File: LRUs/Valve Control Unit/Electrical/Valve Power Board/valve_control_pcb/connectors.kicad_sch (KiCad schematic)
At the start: 21 parts, among them J7 0768290110, J8 Conn_02x10_Odd_Even, U7 TPD6E05U06RVZ, U8 TPD6E05U06RVZ, U9 PCA9306DC

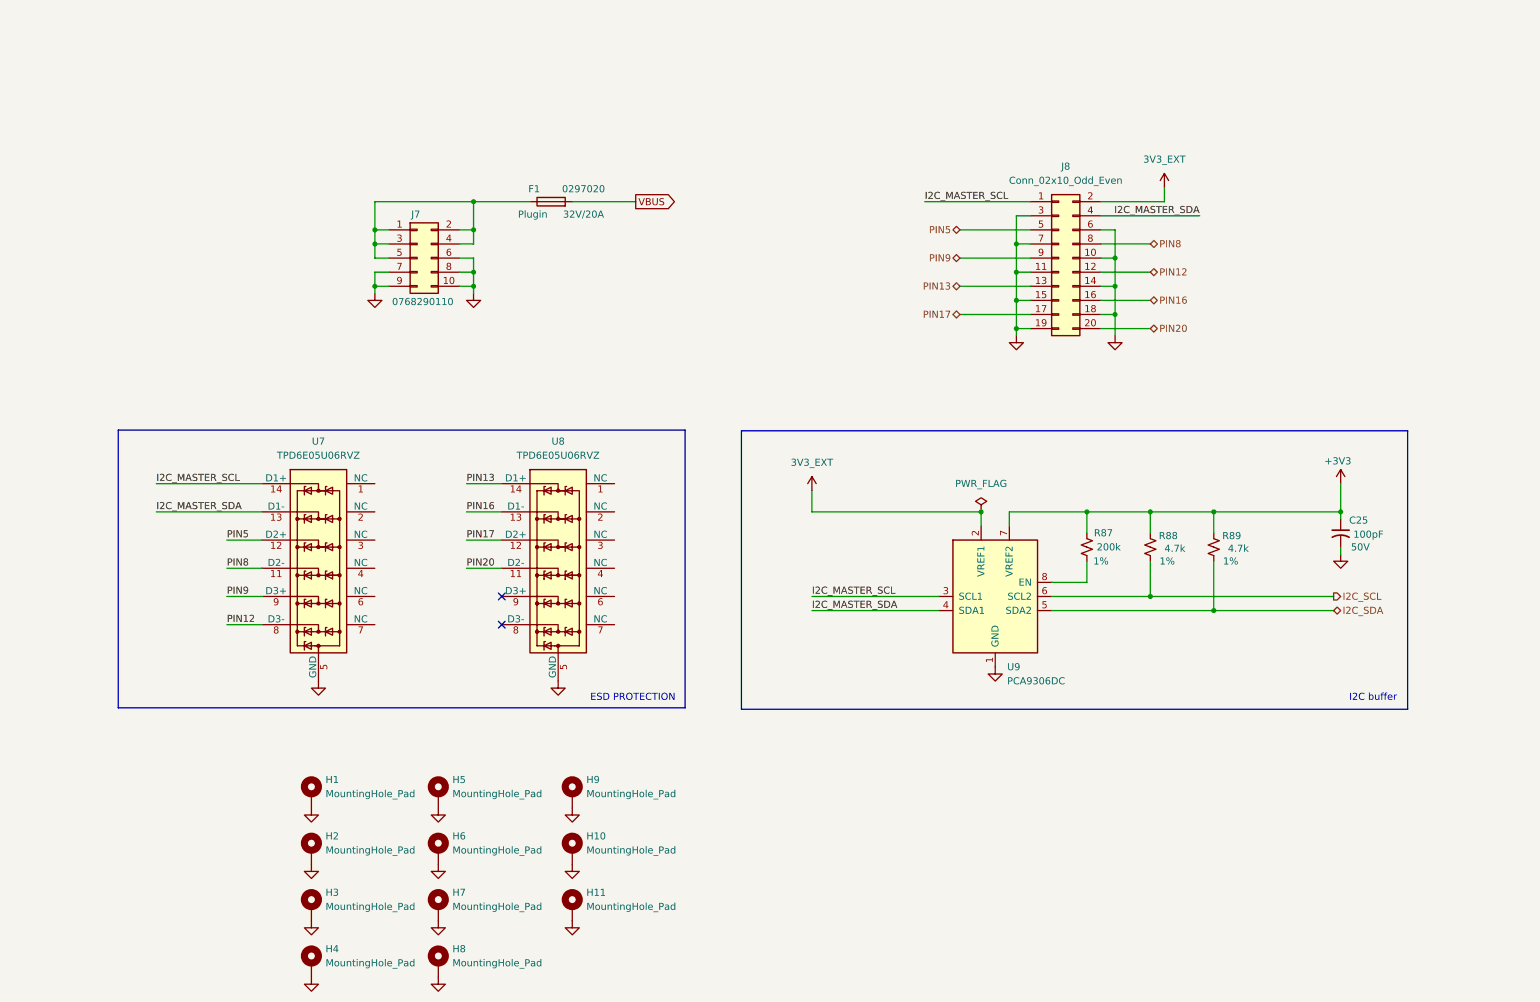
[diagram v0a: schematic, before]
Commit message: Commit valve board updates
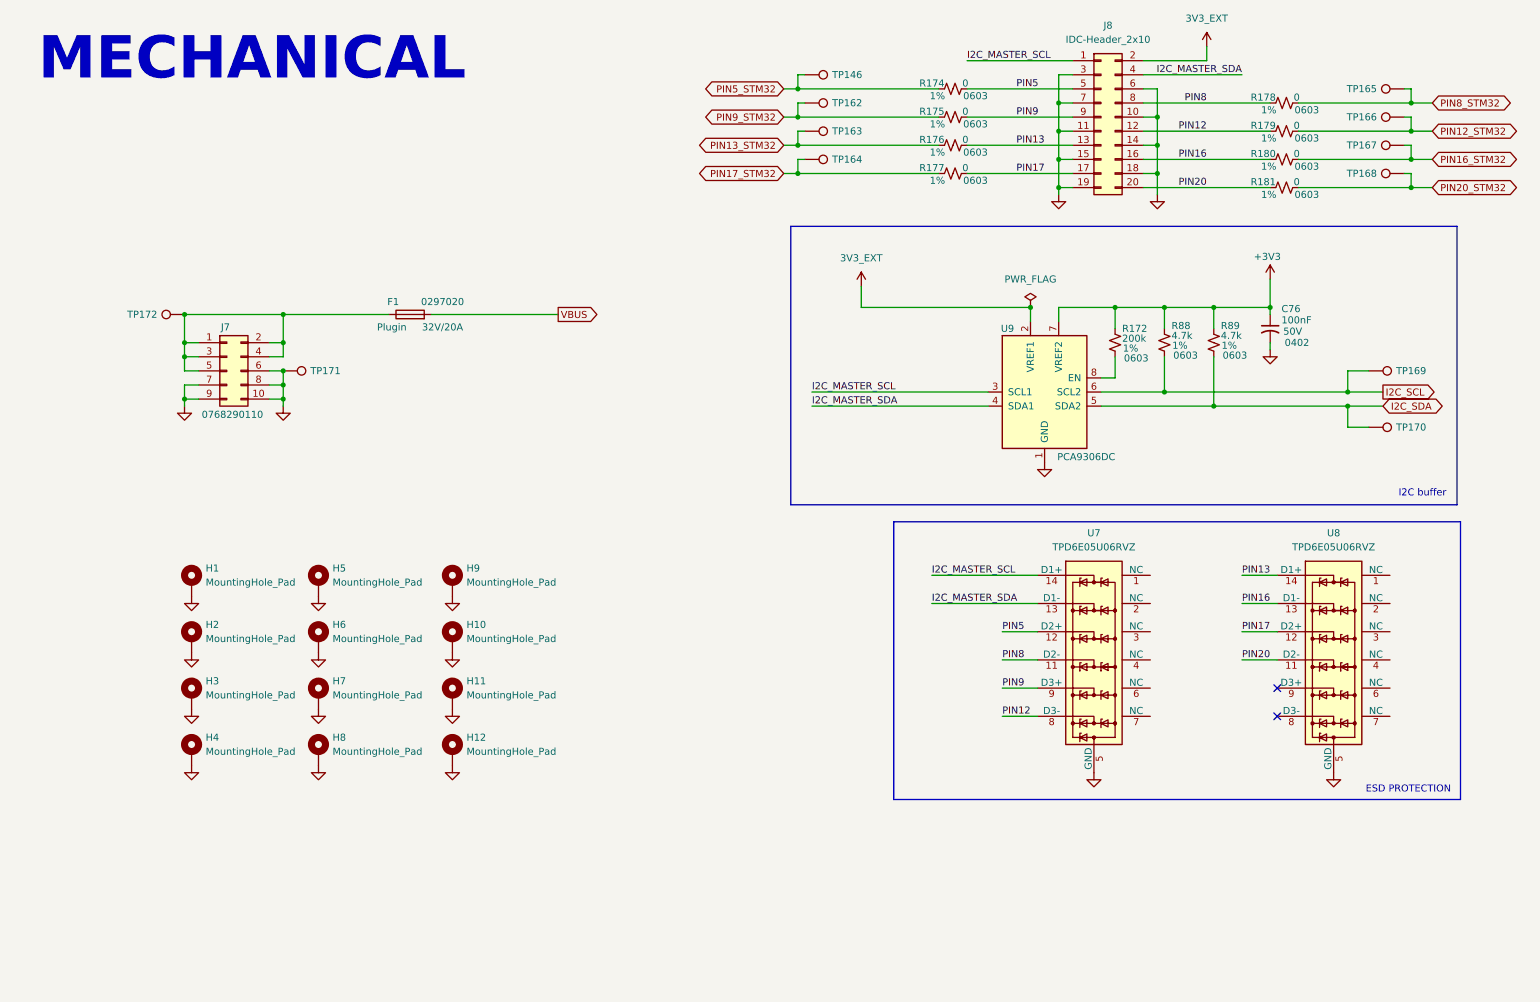
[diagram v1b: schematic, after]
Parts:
- removed C25: 100pF, Capacitor_SMD:C_0402_1005Metric, symbol Device:C_Small_US
- removed R87: 200k, Resistor_SMD:R_0603_1608Metric, symbol Device:R_Small_US
- added C76: 100nF, Capacitor_SMD:C_0402_1005Metric, symbol Device:C_Small_US
- added H12: MountingHole_Pad, MountingHole:MountingHole_3.2mm_M3_ISO14580_Pad, symbol Mechanical:MountingHole_Pad
- added R172: 200k, Resistor_SMD:R_0603_1608Metric, symbol Device:R_Small_US
- added R174, R175, R176, R177, R178, R179, R180, R181: 0, Resistor_SMD:R_0603_1608Metric, symbol Device:R_Small_US
- added TP146, TP162, TP163, TP164, TP165, TP166, TP167, TP168, TP169, TP170, TP171, TP172: TestPoint, TestPoint:TestPoint_Pad_D2.0mm, symbol Connector:TestPoint
- J8: value Conn_02x10_Odd_Even -> IDC-Header_2x10
- R88, R89: Footprint_Size (none) -> 0603
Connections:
- net +3V3: now also C76.1, R172.2
- net GND: now also C76.2, H12.1, TP171.1
- net I2C_SCL: now also TP169.1
- net I2C_SDA: now also TP170.1
- net PIN12: now also R179.2
- net PIN13: now also R176.1
- net PIN16: now also R180.2
- net PIN17: now also R177.1
- net PIN20: now also R181.2
- net PIN5: now also R174.1
- net PIN8: now also R178.2
- net PIN9: now also R175.1
- net at U9.8 (EN): now also R172.1
- net at F1.1, J7.1 (Pin_1), J7.2 (Pin_2)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: now also TP172.1
- new net PIN12_STM32: R179.1, TP166.1
- new net PIN13_STM32: R176.2, TP163.1
- new net PIN16_STM32: R180.1, TP167.1
- new net PIN17_STM32: R177.2, TP164.1
- new net PIN20_STM32: R181.1, TP168.1
- new net PIN5_STM32: R174.2, TP146.1
- new net PIN8_STM32: R178.1, TP165.1
- new net PIN9_STM32: R175.2, TP162.1
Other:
- note added: "MECHANICAL"
- title: (none) -> MECHANICAL
- moved on the sheet: F1, H1, H10, H11, H2, H3, H4, H5, H6, H7, H8, H9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
